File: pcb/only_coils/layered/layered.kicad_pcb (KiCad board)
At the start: 4 copper layers, 70 x 50 mm, 8 parts, among them J2 Conn_01x06_Pin, J4 Conn_01x03_Pin

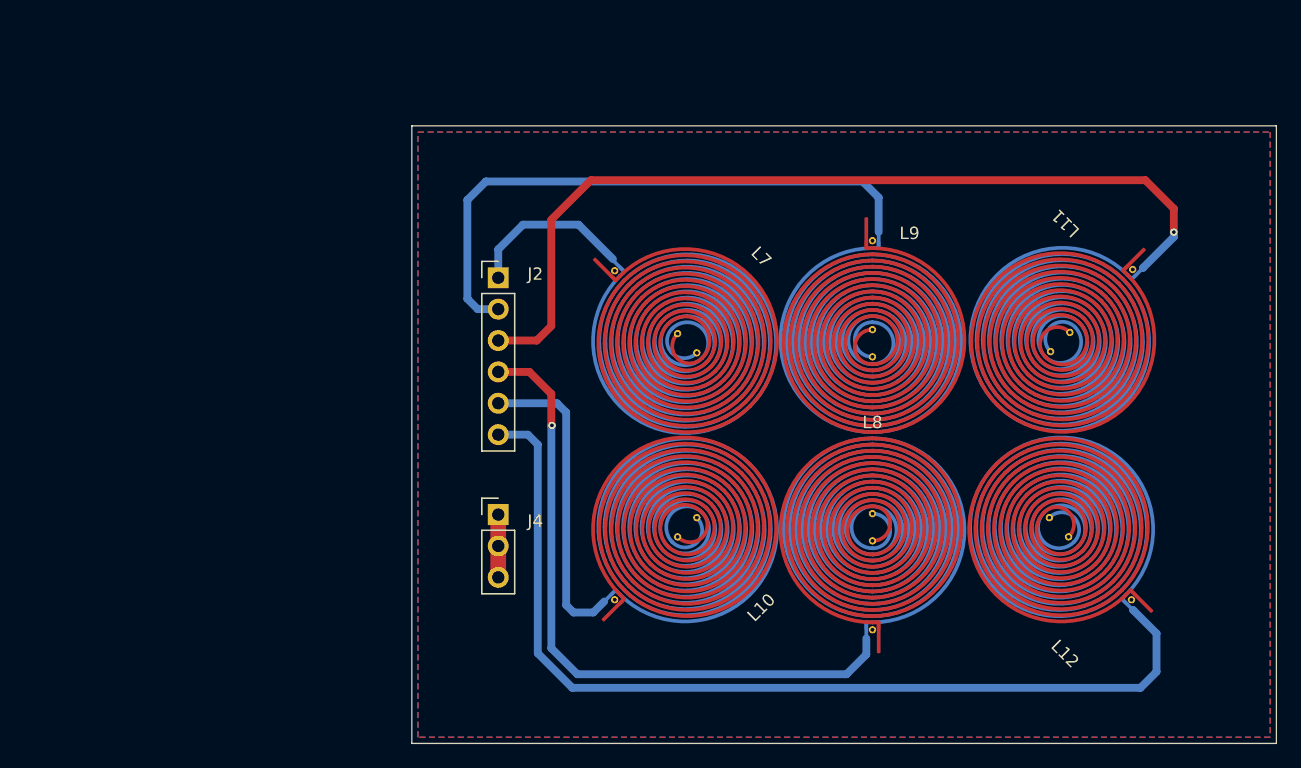
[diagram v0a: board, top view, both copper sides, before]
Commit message: Added  finished layered PCB
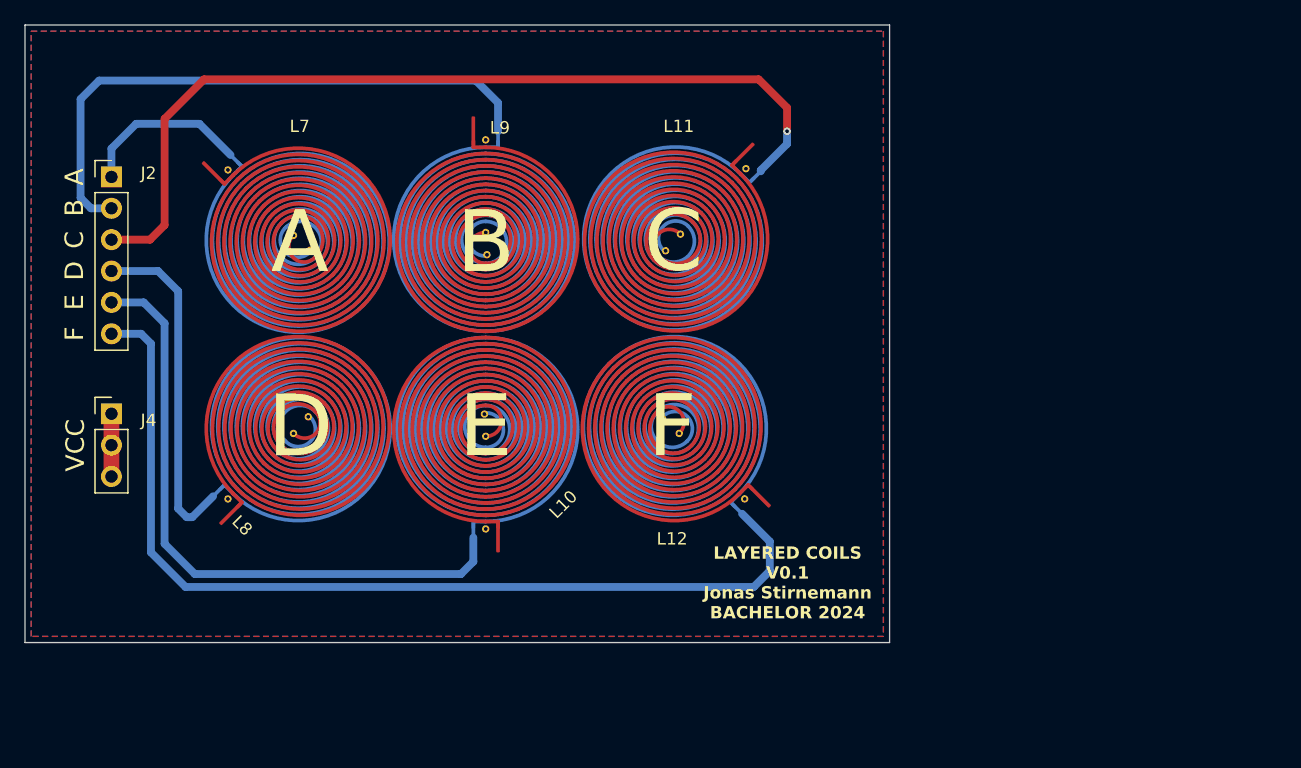
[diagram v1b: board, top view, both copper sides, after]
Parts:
- moved L8 47.0 mm to (89.0, 67.3), turned to -135 degrees
- moved L9 32.4 mm to (104.0, 52.4)
- moved L11 32.4 mm to (119.2, 52.3)
- moved L7 32.4 mm to (89.0, 52.4)
- moved J2 32.4 mm to (73.7, 47.1)
- moved J4 32.4 mm to (73.7, 66.3)
- moved L12 32.4 mm to (119.1, 67.3)
- moved L10 18.2 mm to (104.0, 67.3), turned to -90 degrees
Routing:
- net /D: track 54.0 -> 27.5 mm, vias 1 -> 0
- net /E: track 25.1 -> 51.2 mm
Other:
- board text added: "A"
- board text added: "B"
- board text added: "C"
- board text added: "D"
- board text added: "E"
- board text added: "F"
- board text added: "LAYERED COILS V0.1 Jonas Stirnemann BACHELOR 2024"
- board text added: "LAYERED MODULE - 4 layer coils - 12 turns / layer - 11 mils traces - 10 mils gap"
- board text added: "VCC"
